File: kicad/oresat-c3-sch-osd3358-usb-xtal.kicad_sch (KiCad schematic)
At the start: 36 parts, among them U1 OSD3358-512M-BSM, U11 RCLAMP0504FB, Y1 24MHz, Y2 Crystal

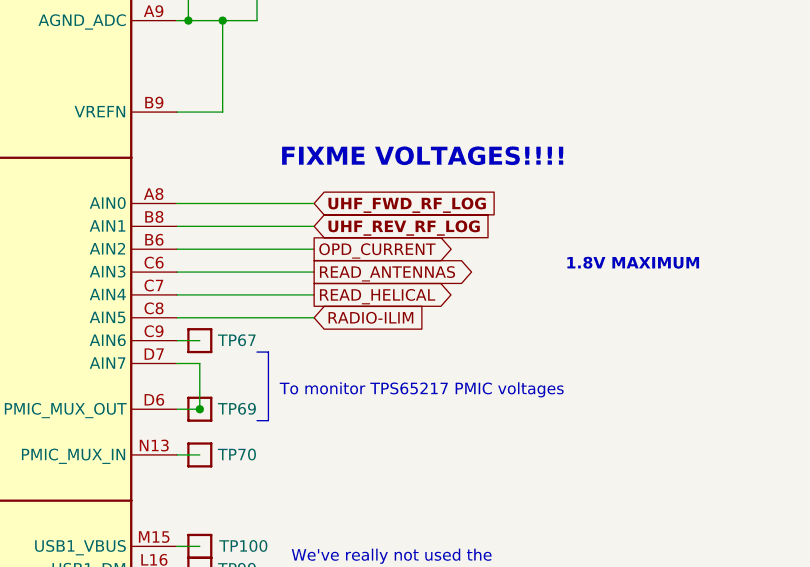
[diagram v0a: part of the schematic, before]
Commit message: Zero airwires! Rough draft schematic and layout are done. Still need ERC and DRC and full design review and stiching and polish.
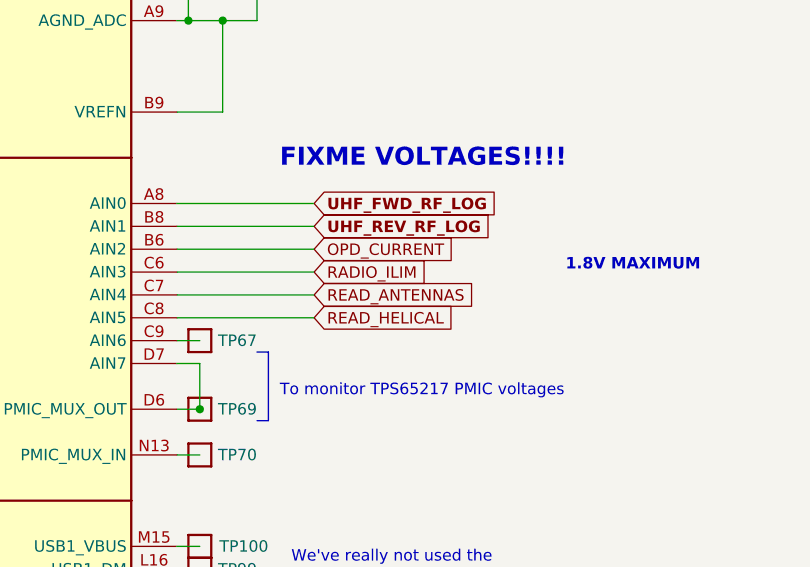
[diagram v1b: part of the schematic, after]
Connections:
- net RADIO-ILIM is gone; now on net READ_HELICAL: U1.C8 (AIN5)
- net READ_ANTENNAS: now also U1.C7 (AIN4); no longer U1.C6 (AIN3)
- net READ_HELICAL: no longer U1.C7 (AIN4)
- new net RADIO_ILIM: U1.C6 (AIN3)
